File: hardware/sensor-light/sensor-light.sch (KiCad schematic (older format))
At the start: 17 parts, among them J1 Power IN 12V, J2 PIR Sensor 2, J3 PIR Sensor 1, J4 PROG Header, J5 Light Sensor, J6 PWM Power OUT 12V, Q1 IRLML2502, SW1 Manual ON/OFF, U1 Reg 3.3V, U2 MSP430G2553IN20

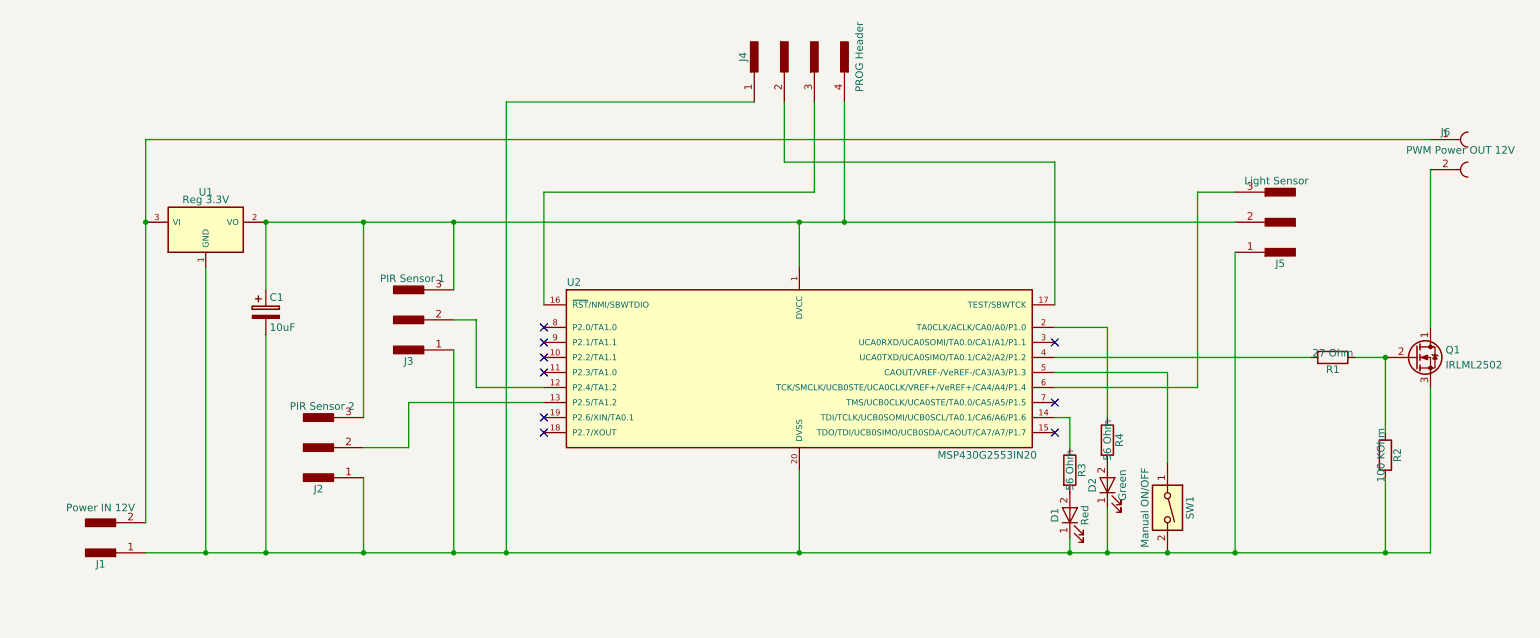
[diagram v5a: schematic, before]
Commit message: some attempt of pcb routing
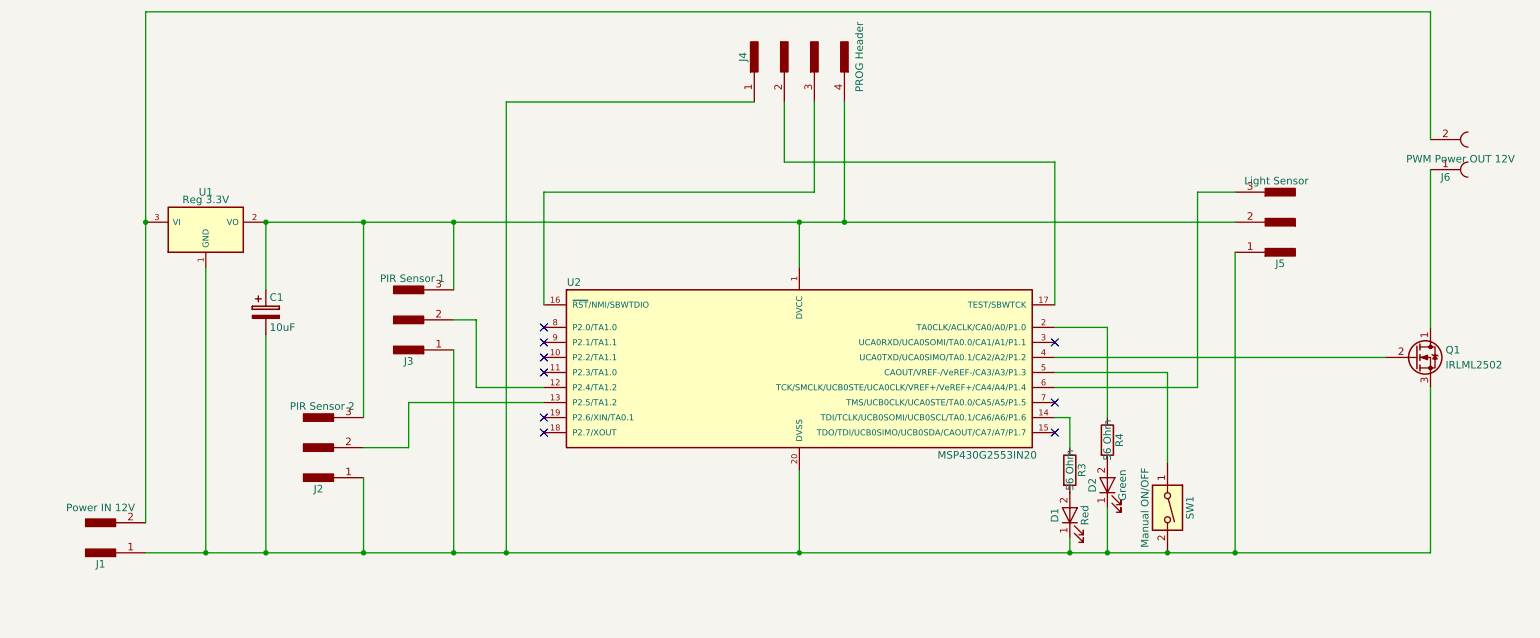
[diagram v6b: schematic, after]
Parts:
- removed R1: 27 Ohm, Resistors_THT:R_Axial_DIN0411_L9.9mm_D3.6mm_P12.70mm_Horizontal, symbol R
- removed R2: 100 KOhm, Resistors_THT:R_Axial_DIN0411_L9.9mm_D3.6mm_P12.70mm_Horizontal, symbol R
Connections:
- net at U2.4 (UCA0TXD/UCA0SIMO/TA0.1/CA2/A2/P1.2): now also Q1.2 (G)
- net at J1.2, U1.3 (VI): now also J6.2; no longer J6.1
- net at Q1.1 (D): now also J6.1; no longer J6.2
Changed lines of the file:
@@
-$EndComp
-$Comp
-L R R2
-U 1 1 5A4A4D3B
-P 9650 4850
-F 0 "R2" V 9730 4850 50  0000 C CNN
-F 1 "100 KOhm" V 9650 4850 50  0000 C BNN
-F 2 "Resistors_THT:R_Axial_DIN0411_L9.9mm_D3.6mm_P12.70mm_Horizontal" V 9580 4850 50  0001 C CNN
-F 3 "" H 9650 4850 50  0001 C CNN
-	1    9650 4850
-	1    0    0    -1
-$EndComp
-$Comp
-L R R1
-U 1 1 5A4A4DD8
-P 9300 4200
-F 0 "R1" V 9380 4200 50  0000 C CNN
-F 1 "27 Ohm" V 9300 4200 50  0000 C BNN
-F 2 "Resistors_THT:R_Axial_DIN0411_L9.9mm_D3.6mm_P12.70mm_Horizontal" V 9230 4200 50  0001 C CNN
-F 3 "" H 9300 4200 50  0001 C CNN
-	1    9300 4200
-	0    1    1    0
 $EndComp
 $Comp
@@
 F 3 "" H 10050 2850 50  0001 C CNN
 	1    10050 2850
-	1    0    0    -1
+	1    0    0    1
 $EndComp
 $Comp
@@
 Connection ~ 1800 5500
 Wire Wire Line
-	1400 2750 1400 5300
-Wire Wire Line
-	1400 2750 9950 2750
+	1400 1900 1400 5300
+Wire Wire Line
+	1400 1900 9950 1900
 Connection ~ 1400 3300
 Wire Wire Line
@@
 Connection ~ 2200 5500
 Connection ~ 2200 3300
-Wire Wire Line
-	9650 4200 9650 4700
-Wire Wire Line
-	9650 5000 9650 5500
-Connection ~ 9650 5500
-Connection ~ 9650 4200
 Connection ~ 5750 5500
 Wire Wire Line
@@
 Connection ~ 8650 5500
 Wire Wire Line
-	9450 4200 9650 4200
-Wire Wire Line
-	9150 4200 7450 4200
+	7450 4200 9650 4200
 Connection ~ 8200 5500
 Wire Wire Line
@@
 Wire Wire Line
 	7550 4800 7550 4600
+Wire Wire Line
+	9950 1900 9950 2750
 $EndSCHEMATC

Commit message: correct MOSFET pinout
Signed-off-by: Eugene Crosser <evgenii.cherkashin@profitbricks.com>
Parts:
- D1, D2: symbol LED -> LED-RESCUE-sensor-light
- Q1: symbol Q_NMOS_DGS -> Q_NMOS_GSD
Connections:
- net at C1.2, D1.1 (K), D2.1 (K)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: now also Q1.2 (S); no longer Q1.3 (S)
- net at U2.4 (UCA0TXD/UCA0SIMO/TA0.1/CA2/A2/P1.2): now also Q1.1 (G); no longer Q1.2 (G)
- net at J6.1: now also Q1.3 (D); no longer Q1.1 (D)
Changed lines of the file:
@@
 $EndComp
 $Comp
-L Q_NMOS_DGS Q1
+L Q_NMOS_GSD Q1
 U 1 1 5A4A4F0F
 P 9850 4200
@@
 $EndComp
 $Comp
-L LED D2
+L LED-RESCUE-sensor-light D2
 U 1 1 5A4A52F3
 P 7800 5050
@@
 $EndComp
 $Comp
-L LED D1
+L LED-RESCUE-sensor-light D1
 U 1 1 5A4A535C
 P 7550 5250
